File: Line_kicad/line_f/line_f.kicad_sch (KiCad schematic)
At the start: 16 parts, among them M2 Motor_DC, M3 Motor_DC, SW1 SW_SPST, SW2 SW_SPDT, SW3 SW_Push, SW4 SW_Push, U1 TB6612FNG_LINE, m1 BLACKPILL

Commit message: 3#
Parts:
- BT1: footprint Connector_AMASS:AMASS_XT60-M_1x02_P7.20mm_Vertical -> LINE_F_FOOT_LIB:BATTERY_LINE_XT60
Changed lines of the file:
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@@
 			)
 		)
-		(property "Footprint" "Connector_AMASS:AMASS_XT60-M_1x02_P7.20mm_Vertical"
+		(property "Footprint" "LINE_F_FOOT_LIB:BATTERY_LINE_XT60"
 			(at 81.026 121.92 90)
 			(effects

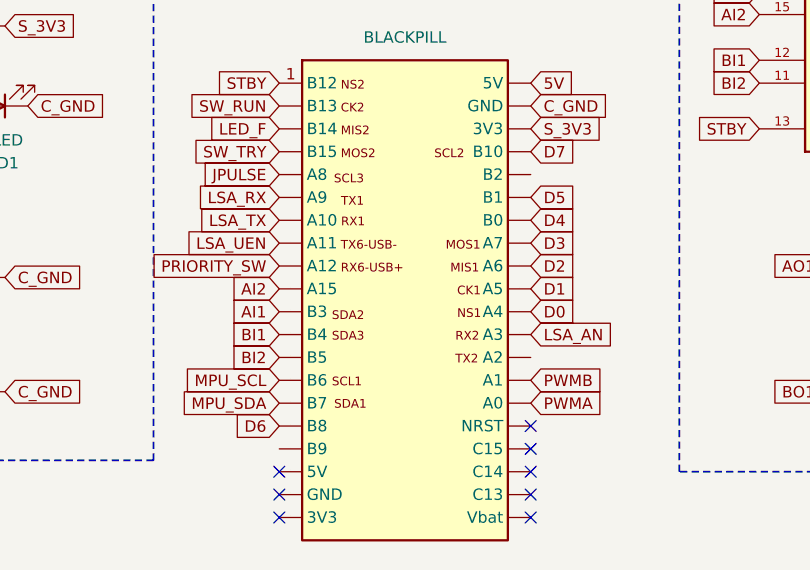
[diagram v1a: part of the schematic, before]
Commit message: 3#
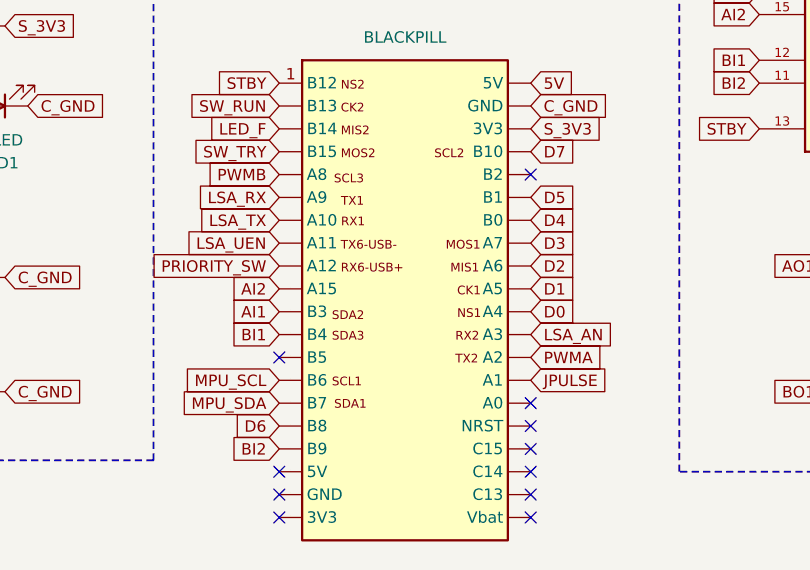
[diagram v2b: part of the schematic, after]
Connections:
- net BI2: now also m1.17 (B9); no longer m1.13 (B5)
- net JPULSE: now also m1.34 (A1); no longer m1.5 (A8)
- net PWMA: now also m1.33 (A2); no longer m1.35 (A0)
- net PWMB: now also m1.5 (A8); no longer m1.34 (A1)
- no-connect marks 10 -> 13
